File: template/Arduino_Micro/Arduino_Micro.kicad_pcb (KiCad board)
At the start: 2 copper layers, 17.8 x 43.2 mm, 6 parts, among them P1 Digital, P2 Analog, P3 CONN_1, P4 CONN_1, P5 CONN_1, P6 CONN_1

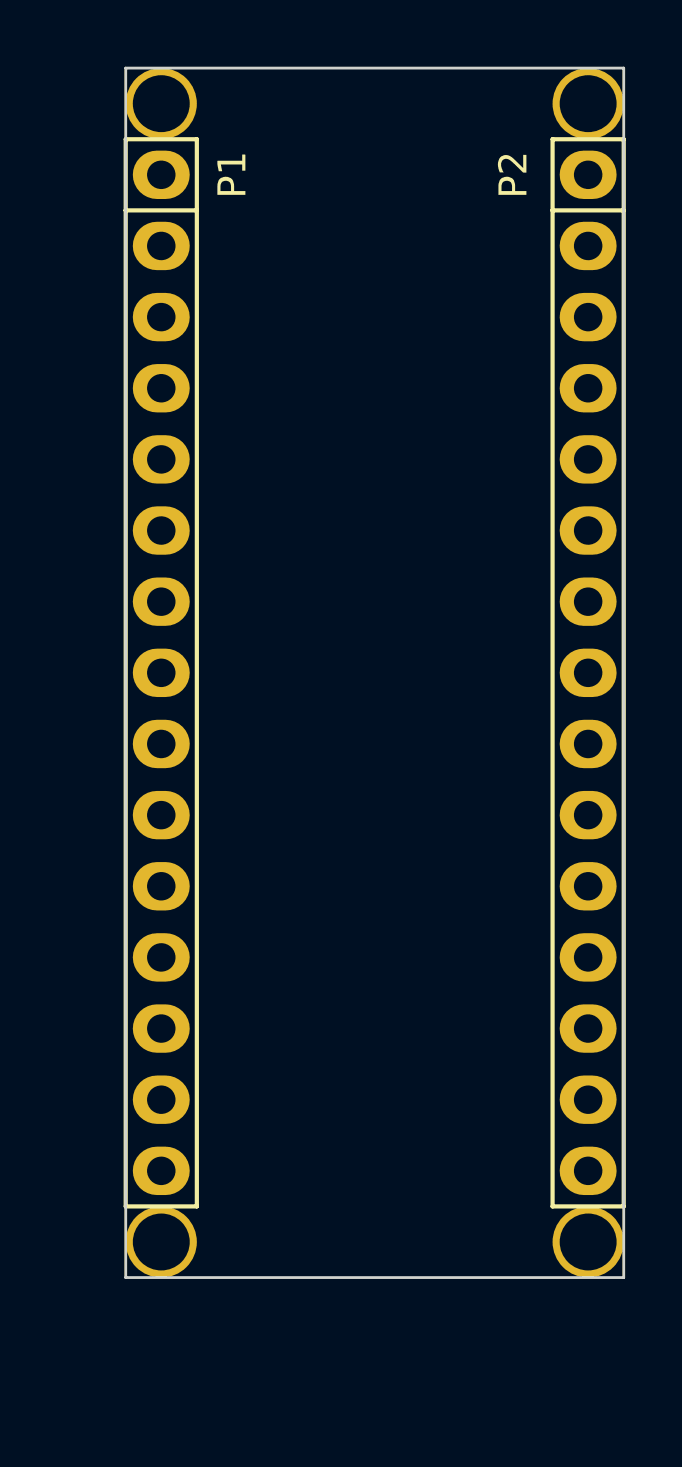
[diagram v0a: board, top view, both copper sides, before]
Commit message: add board Micro
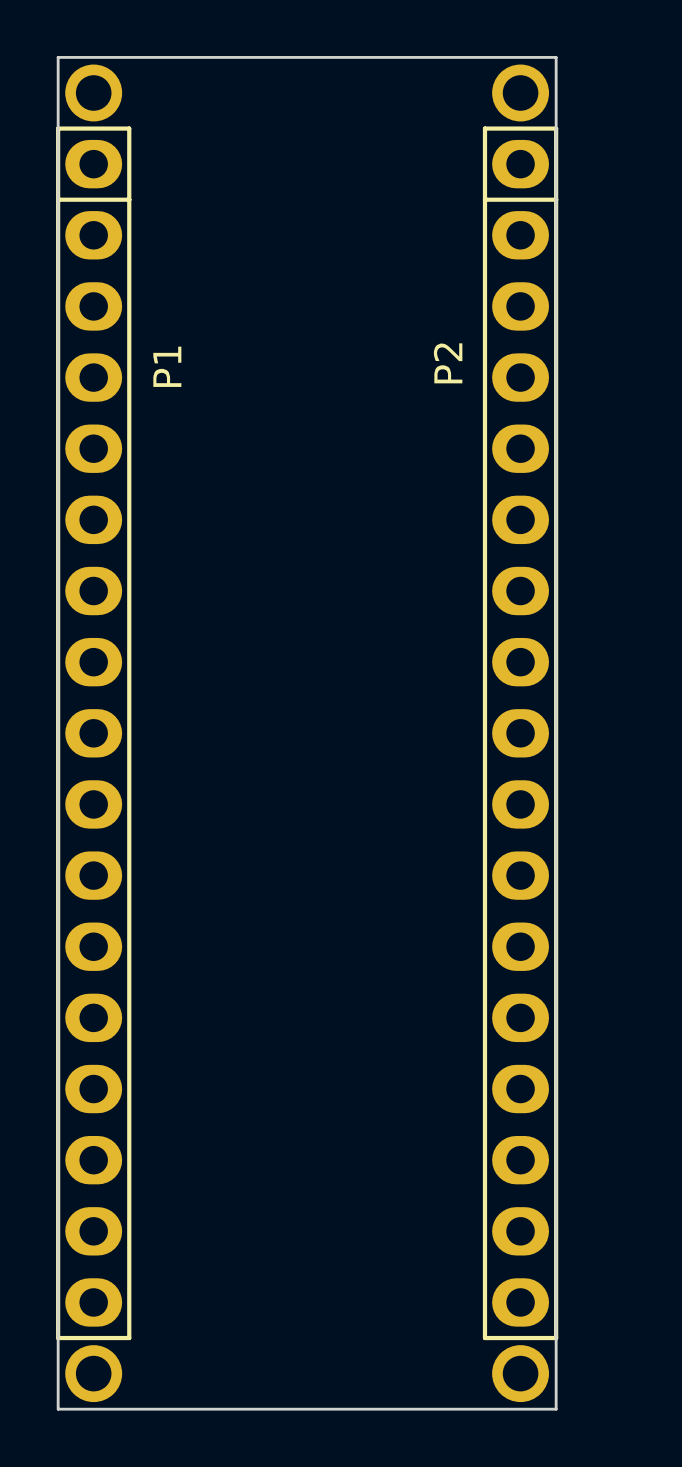
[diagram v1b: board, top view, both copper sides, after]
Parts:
- P1, P2: footprint Socket_Arduino_Nano:Socket_Strip_Arduino_1x15 -> Socket_Arduino_Micro:Socket_Strip_Arduino_1x17
- P3, P4, P5, P6: footprint Socket_Arduino_Nano:1pin_Nano -> Socket_Arduino_Micro:1pin_Micro
- moved P4 5.28 mm to (137.0, 114.0)
- moved P5 5.28 mm to (152.3, 114.0)
- moved P1 2.44 mm to (137.0, 70.9)
- moved P2 2.44 mm to (152.3, 70.9)
- moved P3 2.44 mm to (137.0, 68.3)
- moved P6 2.44 mm to (152.3, 68.3)
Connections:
- net /10(**/SS) renamed /8(A8)
- net /11(**/MISO) renamed /9(**/A9)
- net /12(MOSI) renamed /10(A10)
- net /4 renamed /2(SDA)
- net /6(**) renamed /4(A6)
- net /8 renamed /6(**/A7)
- P1 pad 1: /1(Tx) -> /MOSI
- P1 pad 10: /7 -> /5(**)
- P1 pad 12: /9(**) -> /7
- P1 pad 2: /0(Rx) -> /SS
- P1 pad 3: /Reset -> /1(Tx)
- P1 pad 4: GND -> /0(Rx)
- P1 pad 5: /2 -> /Reset
- P1 pad 6: /3(**) -> GND
- P1 pad 8: /5(**) -> /3(**/SCL)
- P2 pad 1: /Vin -> /SCK
- P2 pad 10: /A2 -> /A4
- P2 pad 11: /A1 -> /A3
- P2 pad 12: /A0 -> /A2
- P2 pad 13: /AREF -> /A1
- P2 pad 14: +3.3V -> /A0
- P2 pad 15: /13(SCK) -> /AREF
- P2 pad 2: GND -> /MISO
- P2 pad 3: /Reset -> /Vin
- P2 pad 4: +5V -> GND
- P2 pad 5: /A7 -> /Reset
- P2 pad 6: /A6 -> +5V
- P2 pad 7: /A5 -> /NC
- P2 pad 8: /A4 -> /NC
- P2 pad 9: /A3 -> /A5
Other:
- board size 17.8 x 43.2 mm -> 17.8 x 48.3 mm

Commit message: corrections
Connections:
- net +3.3V renamed +3V3
- net /0(Rx) renamed /0(Rx1)
- net /1(Tx) renamed /1(Tx1)
- P2 pad 7: /NC -> Net-(P2-Pad7)
- P2 pad 8: /NC -> Net-(P2-Pad8)
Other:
- board text added: "1"
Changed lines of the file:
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@@
 (kicad_pcb (version 4) (host pcbnew "(2015-03-25 BZR 5536)-product")
   (general
-    (links 3)
-    (no_connects 3)
-    (area 135.712999 67.005999 153.593001 115.366001)
+    (links 2)
+    (no_connects 2)
+    (area 133.829429 65.55 155.476572 116.418)
     (thickness 1.6)
-    (drawings 17)
+    (drawings 18)
     (tracks 0)
     (zones 0)
     (modules 6)
-    (nets 36)
+    (nets 37)
   )
   (page A4)
@@
     (mod_text_size 1 1)
     (mod_text_width 0.15)
-    (pad_size 1.5 1.5)
-    (pad_drill 0.6)
+    (pad_size 2.032 2.032)
+    (pad_drill 1.27)
     (pad_to_mask_clearance 0)
     (aux_axis_origin 135.763 115.316)
@@
   (net 1 /MOSI)
   (net 2 /SS)
-  (net 3 "/1(Tx)")
-  (net 4 "/0(Rx)")
-  (net 5 /Reset)
-  (net 6 GND)
-  (net 7 "/2(SDA)")
-  (net 8 "/3(**/SCL)")
-  (net 9 "/4(A6)")
-  (net 10 "/5(**)")
-  (net 11 "/6(**/A7)")
-  (net 12 /7)
-  (net 13 "/8(A8)")
-  (net 14 "/9(**/A9)")
-  (net 15 "/10(A10)")
-  (net 16 "/11(**)")
-  (net 17 "/12(A11)")
-  (net 18 /SCK)
-  (net 19 /MISO)
-  (net 20 /Vin)
-  (net 21 +5V)
-  (net 22 /A5)
-  (net 23 /A4)
-  (net 24 /A3)
-  (net 25 /A2)
-  (net 26 /A1)
-  (net 27 /A0)
-  (net 28 /AREF)
-  (net 29 +3.3V)
-  (net 30 "/13(**)")
-  (net 31 "Net-(P3-Pad1)")
-  (net 32 "Net-(P4-Pad1)")
-  (net 33 "Net-(P5-Pad1)")
-  (net 34 "Net-(P6-Pad1)")
-  (net 35 /NC)
+  (net 3 /Reset)
+  (net 4 GND)
+  (net 5 "/2(SDA)")
+  (net 6 "/3(**/SCL)")
+  (net 7 "/4(A6)")
+  (net 8 "/5(**)")
+  (net 9 "/6(**/A7)")
+  (net 10 /7)
+  (net 11 "/8(A8)")
+  (net 12 "/9(**/A9)")
+  (net 13 "/10(A10)")
+  (net 14 "/11(**)")
+  (net 15 "/12(A11)")
+  (net 16 /SCK)
+  (net 17 /MISO)
+  (net 18 /Vin)
+  (net 19 +5V)
+  (net 20 /A5)
+  (net 21 /A4)
+  (net 22 /A3)
+  (net 23 /A2)
+  (net 24 /A1)
+  (net 25 /A0)
+  (net 26 /AREF)
+  (net 27 "/13(**)")
+  (net 28 "Net-(P3-Pad1)")
+  (net 29 "Net-(P4-Pad1)")
+  (net 30 "Net-(P5-Pad1)")
+  (net 31 "Net-(P6-Pad1)")
+  (net 32 "/1(Tx1)")
+  (net 33 "/0(Rx1)")
+  (net 34 "Net-(P2-Pad7)")
+  (net 35 "Net-(P2-Pad8)")
+  (net 36 +3V3)
   (net_class Default "This is the default net class."
     (clearance 0.2)
@@
     (uvia_dia 0.3)
     (uvia_drill 0.1)
-    (add_net +3.3V)
+    (add_net +3V3)
     (add_net +5V)
-    (add_net "/0(Rx)")
-    (add_net "/1(Tx)")
+    (add_net "/0(Rx1)")
+    (add_net "/1(Tx1)")
     (add_net "/10(A10)")
     (add_net "/11(**)")
@@
     (add_net /MISO)
     (add_net /MOSI)
-    (add_net /NC)
     (add_net /Reset)
     (add_net /SCK)
@@
     (add_net /Vin)
     (add_net GND)
+    (add_net "Net-(P2-Pad7)")
+    (add_net "Net-(P2-Pad8)")
     (add_net "Net-(P3-Pad1)")
     (add_net "Net-(P4-Pad1)")
@@
       (net 2 /SS))
     (pad 3 thru_hole oval (at 5.08 0 270) (size 1.7272 2.032) (drill 1.016) (layers *.Cu *.Mask F.SilkS)
-      (net 3 "/1(Tx)"))
+      (net 32 "/1(Tx1)"))
     (pad 4 thru_hole oval (at 7.62 0 270) (size 1.7272 2.032) (drill 1.016) (layers *.Cu *.Mask F.SilkS)
-      (net 4 "/0(Rx)"))
+      (net 33 "/0(Rx1)"))
     (pad 5 thru_hole oval (at 10.16 0 270) (size 1.7272 2.032) (drill 1.016) (layers *.Cu *.Mask F.SilkS)
-      (net 5 /Reset))
+      (net 3 /Reset))
     (pad 6 thru_hole oval (at 12.7 0 270) (size 1.7272 2.032) (drill 1.016) (layers *.Cu *.Mask F.SilkS)
-      (net 6 GND))
+      (net 4 GND))
     (pad 7 thru_hole oval (at 15.24 0 270) (size 1.7272 2.032) (drill 1.016) (layers *.Cu *.Mask F.SilkS)
-      (net 7 "/2(SDA)"))
+      (net 5 "/2(SDA)"))
     (pad 8 thru_hole oval (at 17.78 0 270) (size 1.7272 2.032) (drill 1.016) (layers *.Cu *.Mask F.SilkS)
-      (net 8 "/3(**/SCL)"))
+      (net 6 "/3(**/SCL)"))
     (pad 9 thru_hole oval (at 20.32 0 270) (size 1.7272 2.032) (drill 1.016) (layers *.Cu *.Mask F.SilkS)
-      (net 9 "/4(A6)"))
+      (net 7 "/4(A6)"))
     (pad 10 thru_hole oval (at 22.86 0 270) (size 1.7272 2.032) (drill 1.016) (layers *.Cu *.Mask F.SilkS)
-      (net 10 "/5(**)"))
+      (net 8 "/5(**)"))
     (pad 11 thru_hole oval (at 25.4 0 270) (size 1.7272 2.032) (drill 1.016) (layers *.Cu *.Mask F.SilkS)
-      (net 11 "/6(**/A7)"))
+      (net 9 "/6(**/A7)"))
     (pad 12 thru_hole oval (at 27.94 0 270) (size 1.7272 2.032) (drill 1.016) (layers *.Cu *.Mask F.SilkS)
-      (net 12 /7))
+      (net 10 /7))
     (pad 13 thru_hole oval (at 30.48 0 270) (size 1.7272 2.032) (drill 1.016) (layers *.Cu *.Mask F.SilkS)
-      (net 13 "/8(A8)"))
+      (net 11 "/8(A8)"))
     (pad 14 thru_hole oval (at 33.02 0 270) (size 1.7272 2.032) (drill 1.016) (layers *.Cu *.Mask F.SilkS)
-      (net 14 "/9(**/A9)"))
+      (net 12 "/9(**/A9)"))
     (pad 15 thru_hole oval (at 35.56 0 270) (size 1.7272 2.032) (drill 1.016) (layers *.Cu *.Mask F.SilkS)
-      (net 15 "/10(A10)"))
+      (net 13 "/10(A10)"))
     (pad 16 thru_hole oval (at 38.1 0 270) (size 1.7272 2.032) (drill 1.016) (layers *.Cu *.Mask F.SilkS)
-      (net 16 "/11(**)"))
+      (net 14 "/11(**)"))
     (pad 17 thru_hole oval (at 40.64 0 270) (size 1.7272 2.032) (drill 1.016) (layers *.Cu *.Mask F.SilkS)
-      (net 17 "/12(A11)"))
-    (model /home/jo/kicad/template/Arduino_Micro/Socket_Arduino_Micro.3dshapes/Socket_header_Arduino_1x17.wrl
+      (net 15 "/12(A11)"))
+    (model ${KIPRJMOD}/Socket_Arduino_Micro.3dshapes/Socket_header_Arduino_1x17.wrl
       (at (xyz 0.8 0 0))
       (scale (xyz 1 1 1))
@@
     (fp_line (start 1.27 1.27) (end 1.27 -1.27) (layer F.SilkS) (width 0.15))
     (pad 1 thru_hole oval (at 0 0 270) (size 1.7272 2.032) (drill 1.016) (layers *.Cu *.Mask F.SilkS)
-      (net 18 /SCK))
+      (net 16 /SCK))
     (pad 2 thru_hole oval (at 2.54 0 270) (size 1.7272 2.032) (drill 1.016) (layers *.Cu *.Mask F.SilkS)
-      (net 19 /MISO))
+      (net 17 /MISO))
     (pad 3 thru_hole oval (at 5.08 0 270) (size 1.7272 2.032) (drill 1.016) (layers *.Cu *.Mask F.SilkS)
-      (net 20 /Vin))
+      (net 18 /Vin))
     (pad 4 thru_hole oval (at 7.62 0 270) (size 1.7272 2.032) (drill 1.016) (layers *.Cu *.Mask F.SilkS)
-      (net 6 GND))
+      (net 4 GND))
     (pad 5 thru_hole oval (at 10.16 0 270) (size 1.7272 2.032) (drill 1.016) (layers *.Cu *.Mask F.SilkS)
-      (net 5 /Reset))
+      (net 3 /Reset))
     (pad 6 thru_hole oval (at 12.7 0 270) (size 1.7272 2.032) (drill 1.016) (layers *.Cu *.Mask F.SilkS)
-      (net 21 +5V))
+      (net 19 +5V))
     (pad 7 thru_hole oval (at 15.24 0 270) (size 1.7272 2.032) (drill 1.016) (layers *.Cu *.Mask F.SilkS)
-      (net 35 /NC))
+      (net 34 "Net-(P2-Pad7)"))
     (pad 8 thru_hole oval (at 17.78 0 270) (size 1.7272 2.032) (drill 1.016) (layers *.Cu *.Mask F.SilkS)
-      (net 35 /NC))
+      (net 35 "Net-(P2-Pad8)"))
     (pad 9 thru_hole oval (at 20.32 0 270) (size 1.7272 2.032) (drill 1.016) (layers *.Cu *.Mask F.SilkS)
-      (net 22 /A5))
+      (net 20 /A5))
     (pad 10 thru_hole oval (at 22.86 0 270) (size 1.7272 2.032) (drill 1.016) (layers *.Cu *.Mask F.SilkS)
-      (net 23 /A4))
+      (net 21 /A4))
     (pad 11 thru_hole oval (at 25.4 0 270) (size 1.7272 2.032) (drill 1.016) (layers *.Cu *.Mask F.SilkS)
-      (net 24 /A3))
+      (net 22 /A3))
     (pad 12 thru_hole oval (at 27.94 0 270) (size 1.7272 2.032) (drill 1.016) (layers *.Cu *.Mask F.SilkS)
-      (net 25 /A2))
+      (net 23 /A2))
     (pad 13 thru_hole oval (at 30.48 0 270) (size 1.7272 2.032) (drill 1.016) (layers *.Cu *.Mask F.SilkS)
-      (net 26 /A1))
+      (net 24 /A1))
     (pad 14 thru_hole oval (at 33.02 0 270) (size 1.7272 2.032) (drill 1.016) (layers *.Cu *.Mask F.SilkS)
-      (net 27 /A0))
+      (net 25 /A0))
     (pad 15 thru_hole oval (at 35.56 0 270) (size 1.7272 2.032) (drill 1.016) (layers *.Cu *.Mask F.SilkS)
-      (net 28 /AREF))
+      (net 26 /AREF))
     (pad 16 thru_hole oval (at 38.1 0 270) (size 1.7272 2.032) (drill 1.016) (layers *.Cu *.Mask F.SilkS)
-      (net 29 +3.3V))
+      (net 36 +3V3))
     (pad 17 thru_hole oval (at 40.64 0 270) (size 1.7272 2.032) (drill 1.016) (layers *.Cu *.Mask F.SilkS)
-      (net 30 "/13(**)"))
-    (model /home/jo/kicad/template/Arduino_Micro/Socket_Arduino_Micro.3dshapes/Socket_header_Arduino_1x17.wrl
+      (net 27 "/13(**)"))
+    (model ${KIPRJMOD}/Socket_Arduino_Micro.3dshapes/Socket_header_Arduino_1x17.wrl
       (at (xyz 0.8 0 0))
       (scale (xyz 1 1 1))
@@
     )
     (pad 1 thru_hole circle (at 0 0) (size 2.032 2.032) (drill 1.27) (layers *.Cu *.Mask F.SilkS)
-      (net 31 "Net-(P3-Pad1)"))
+      (net 28 "Net-(P3-Pad1)"))
   )
   (module Socket_Arduino_Micro:1pin_Micro (layer F.Cu)
@@
     )
     (pad 1 thru_hole circle (at 0 0) (size 2.032 2.032) (drill 1.27) (layers *.Cu *.Mask F.SilkS)
-      (net 32 "Net-(P4-Pad1)"))
+      (net 29 "Net-(P4-Pad1)"))
   )
   (module Socket_Arduino_Micro:1pin_Micro (layer F.Cu)
@@
     )
     (pad 1 thru_hole circle (at 0 0) (size 2.032 2.032) (drill 1.27) (layers *.Cu *.Mask F.SilkS)
-      (net 33 "Net-(P5-Pad1)"))
+      (net 30 "Net-(P5-Pad1)"))
   )
   (module Socket_Arduino_Micro:1pin_Micro (layer F.Cu)
@@
     )
     (pad 1 thru_hole circle (at 0 0) (size 2.032 2.032) (drill 1.27) (layers *.Cu *.Mask F.SilkS)
-      (net 34 "Net-(P6-Pad1)"))
+      (net 31 "Net-(P6-Pad1)"))
+  )
+  (gr_text 1 (at 134.747 70.866) (layer Dwgs.User)
+    (effects (font (size 1.5 1.5) (thickness 0.3)))
   )
   (gr_line (start 141.097 116.078) (end 148.209 116.078) (angle 90) (layer Dwgs.User) (width 0.15))
